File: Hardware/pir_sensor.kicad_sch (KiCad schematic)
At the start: 30 parts, among them U5 D203S, U6 LM358, U7 LM393

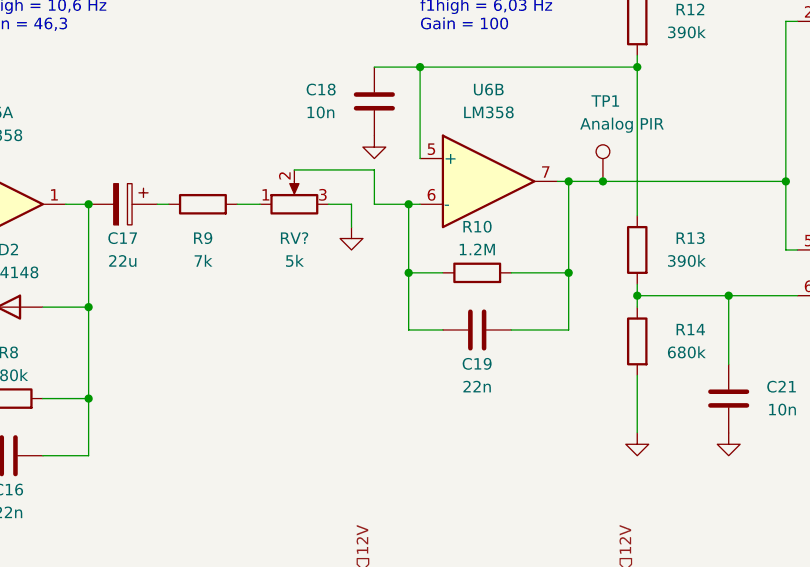
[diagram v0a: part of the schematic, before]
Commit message: v1.2.0. Prototype schematic correction
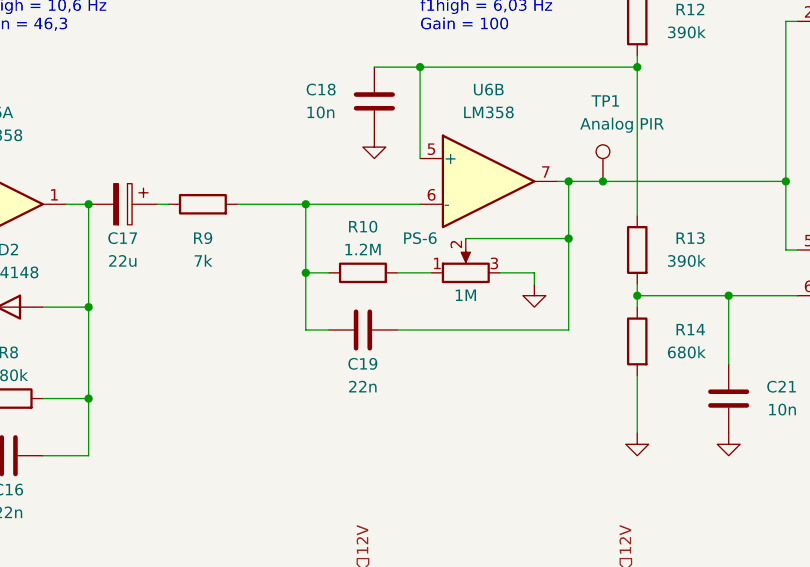
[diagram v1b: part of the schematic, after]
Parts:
- removed RV?: 5k, symbol Device:R_Potentiometer
- added PS-6: 1M, Local:Potentiometer_PS-6_Vertical_Hole, symbol Device:R_Potentiometer
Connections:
- net GND: now also PS-6.3
- net at C19.1, R10.1, U6.6 (-): now also R9.2
- net at C19.2, TP1.1, U6.7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: now also PS-6.2; no longer R10.2
- new net: PS-6.1, R10.2
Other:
- moved on the sheet: C19, R10
